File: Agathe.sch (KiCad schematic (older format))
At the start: 180 parts, among them J1 Conn_01x04_Female, J2 Conn_01x02_Female, J3 AVR-ISP-6, J4 Conn_01x02_Female, SW1 SW_Push, U1 ATmega32U4-AU, U2 PRTR5V0U2X, Y1 16MHz

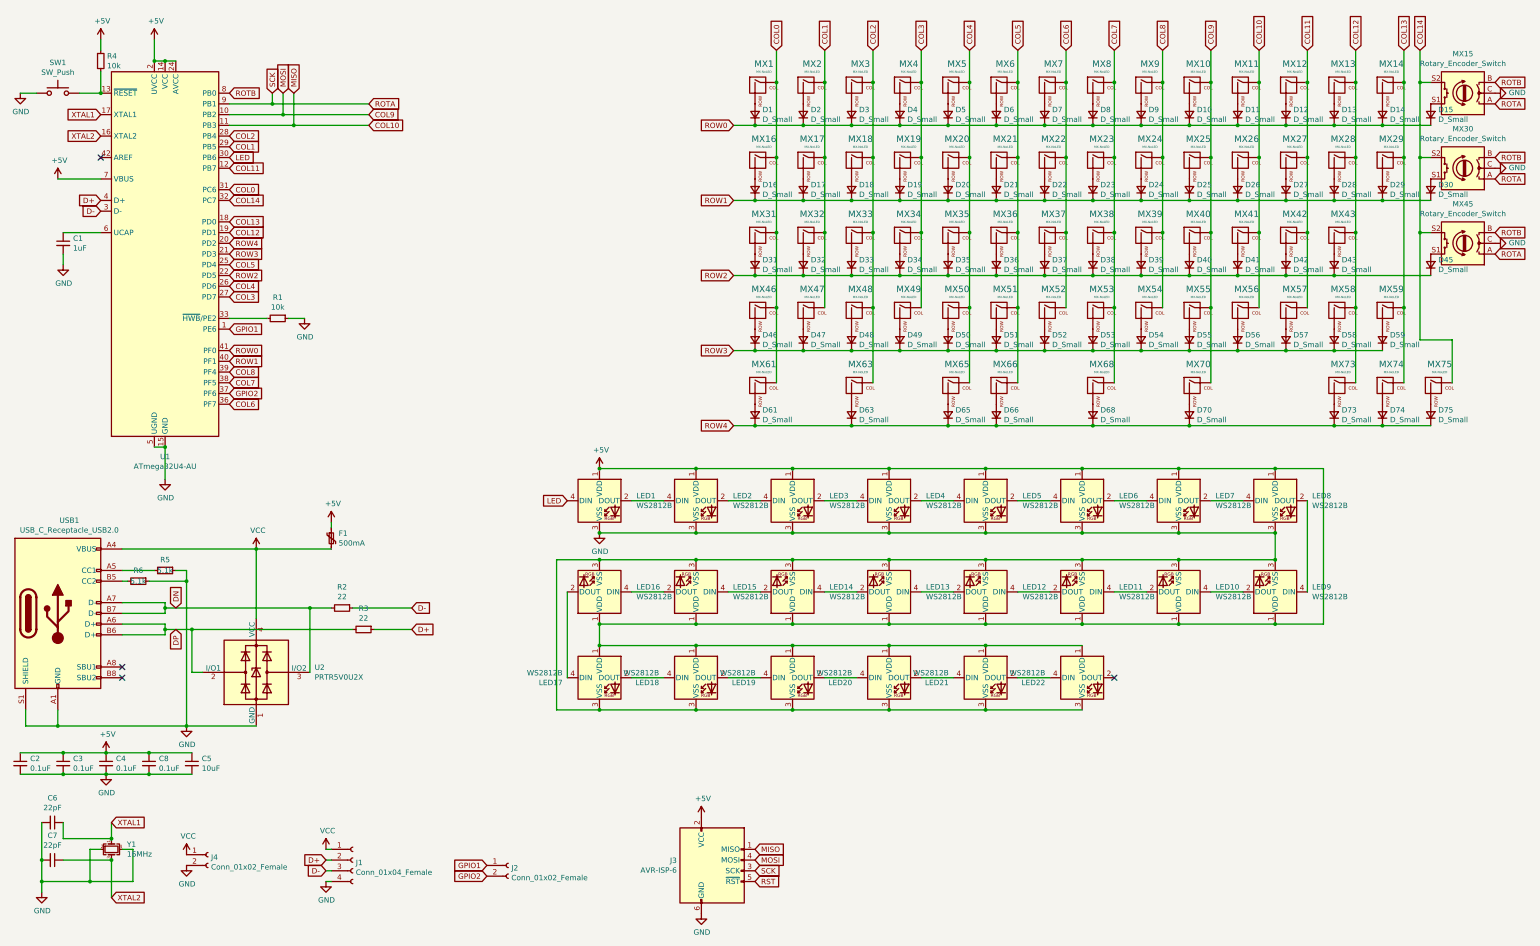
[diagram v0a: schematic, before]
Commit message: j'ai putain de tout refait putain
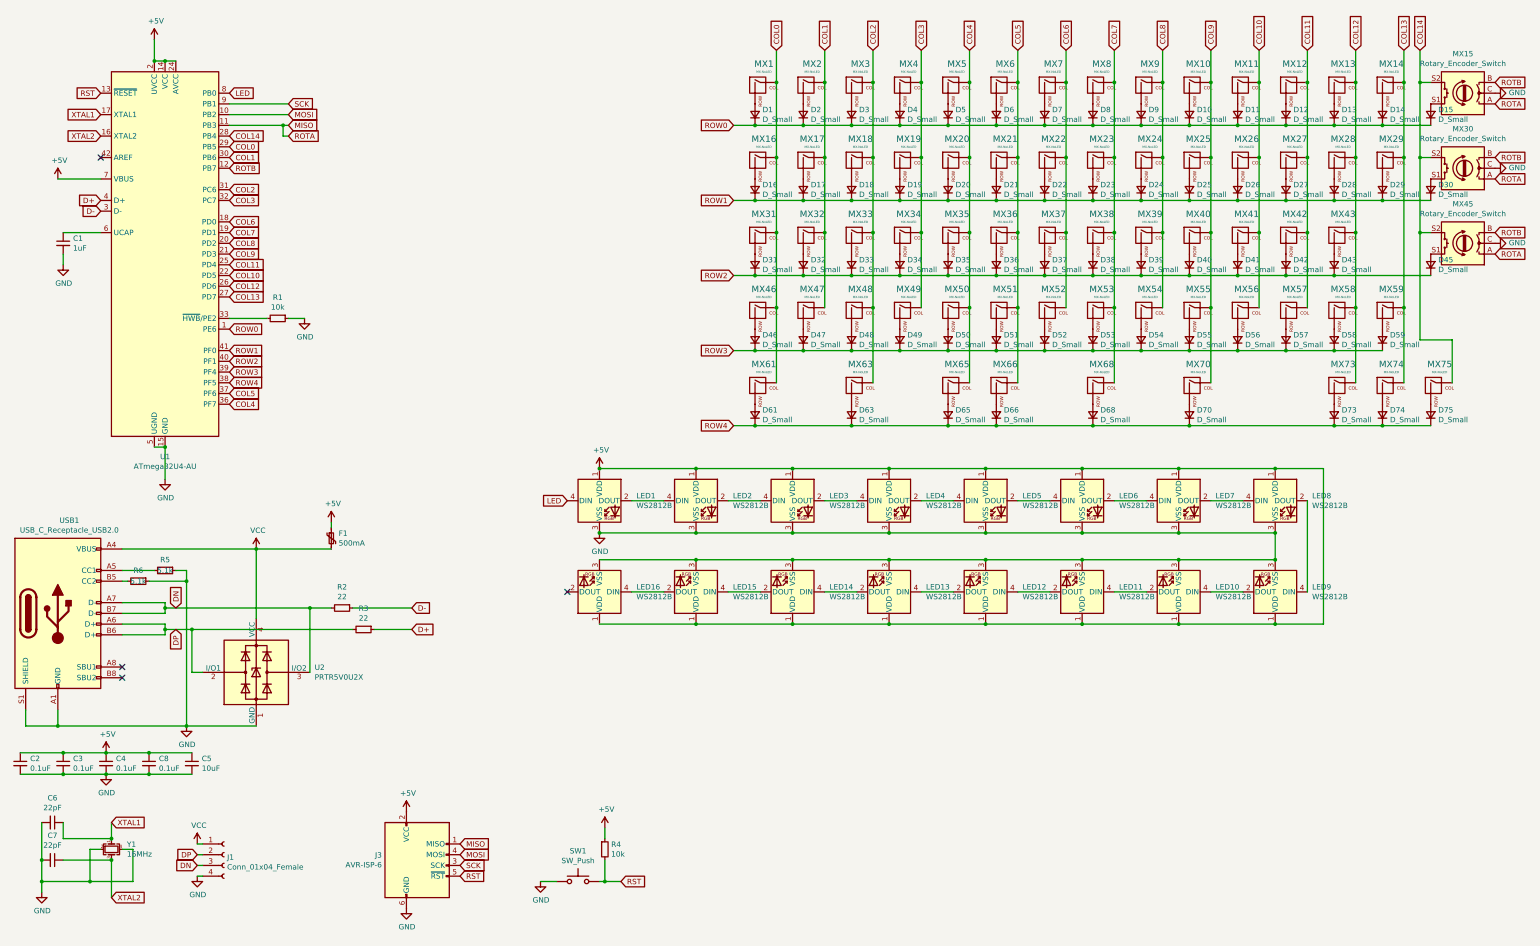
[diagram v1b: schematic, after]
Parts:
- removed J2, J4: Conn_01x02_Female, Connector_PinHeader_2.54mm:PinHeader_1x02_P2.54mm_Vertical, symbol Connector:Conn_01x02_Female
- removed LED17, LED18, LED19, LED20, LED21, LED22: WS2812B, LED_SMD:LED_WS2812B_PLCC4_5.0x5.0mm_P3.2mm, symbol LED:WS2812B
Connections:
- net GPIO1 is gone; now on net ROW0: U1.1 (PE6)
- net GPIO2 is gone; now on net COL5: U1.37 (PF6)
- net COL0: now also U1.29 (PB5); no longer U1.31 (PC6)
- net COL1: now also U1.30 (PB6); no longer U1.29 (PB5)
- net COL10: now also U1.22 (PD5); no longer J3.1 (MISO), U1.11 (PB3)
- net COL11: now also U1.25 (PD4); no longer U1.12 (PB7)
- net COL12: now also U1.26 (PD6); no longer U1.19 (PD1)
- net COL13: now also U1.27 (PD7); no longer U1.18 (PD0)
- net COL14: now also U1.28 (PB4); no longer U1.32 (PC7)
- net COL2: now also U1.31 (PC6); no longer U1.28 (PB4)
- net COL3: now also U1.32 (PC7); no longer U1.27 (PD7)
- net COL4: now also U1.36 (PF7); no longer U1.26 (PD6)
- net COL5: no longer U1.25 (PD4)
- net COL6: now also U1.18 (PD0); no longer U1.36 (PF7)
- net COL7: now also U1.19 (PD1); no longer U1.38 (PF5)
- net COL8: now also U1.20 (PD2); no longer U1.39 (PF4)
- net COL9: now also U1.21 (PD3); no longer J3.4 (MOSI), U1.10 (PB2)
- net D+: no longer J1.2 (Pin_2)
- net D-: no longer J1.3 (Pin_3)
- net DN: now also J1.3 (Pin_3)
- net DP: now also J1.2 (Pin_2)
- net LED: now also U1.8 (PB0); no longer U1.30 (PB6)
- net ROTB: now also U1.12 (PB7); no longer U1.8 (PB0)
- net ROW0: no longer U1.41 (PF0)
- net ROW1: now also U1.41 (PF0); no longer U1.40 (PF1)
- net ROW2: now also U1.40 (PF1); no longer U1.22 (PD5)
- net ROW3: now also U1.39 (PF4); no longer U1.21 (PD3)
- net ROW4: now also U1.38 (PF5); no longer U1.20 (PD2)
- net RST: now also R4.2, SW1.2, U1.13 (~RESET)
- net ROTA renamed MISO
- net MISO: now also J3.1 (MISO), U1.11 (PB3); no longer J3.3 (SCK), U1.9 (PB1)
- new net MOSI: J3.4 (MOSI), U1.10 (PB2)
- new net SCK: J3.3 (SCK), U1.9 (PB1)
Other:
- moved on the sheet: J1, J3, R4, SW1
